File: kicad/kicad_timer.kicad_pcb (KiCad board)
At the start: 2 copper layers, 70.8 x 70.8 mm, 18 parts, among them J1 USB_C_Receptacle_PowerOnly_6P, U1 CA56-12CGKWA, U2 ATmega328-A, U3 CA56-12CGKWA

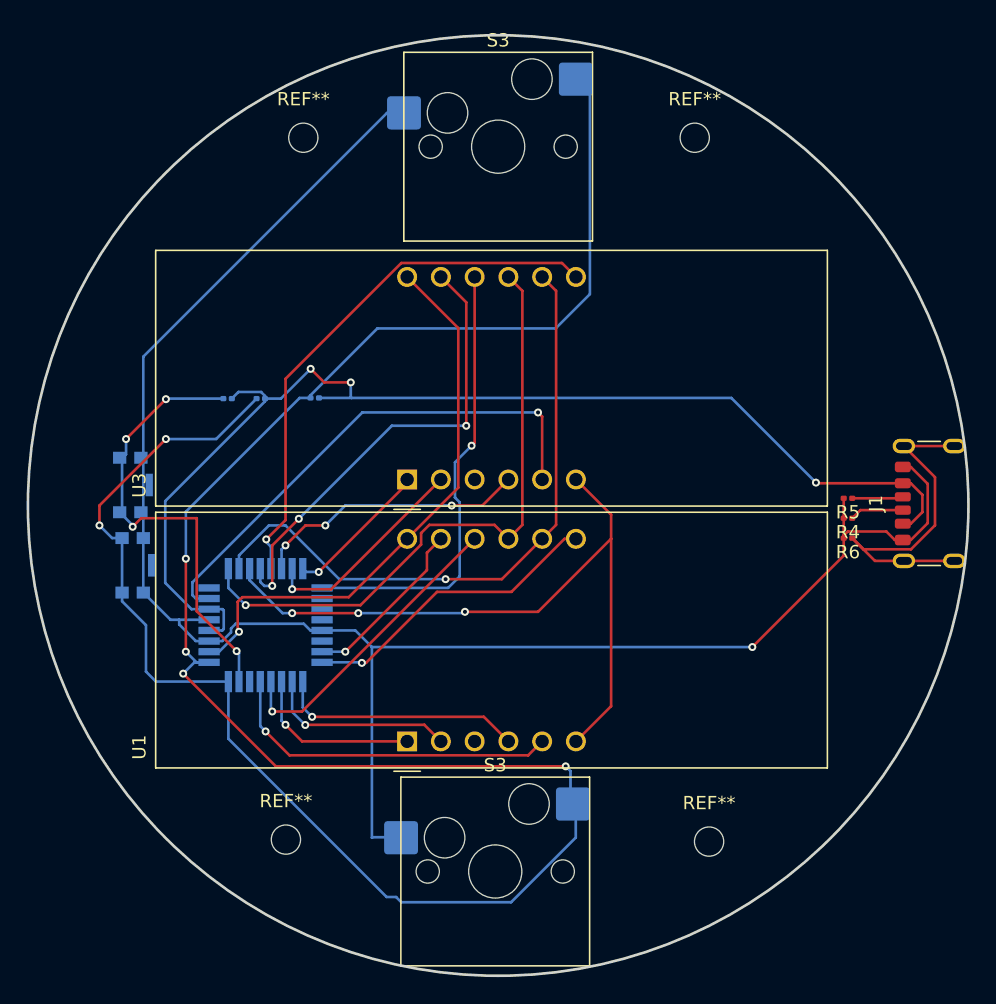
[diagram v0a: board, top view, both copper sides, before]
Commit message: Improving the pcb
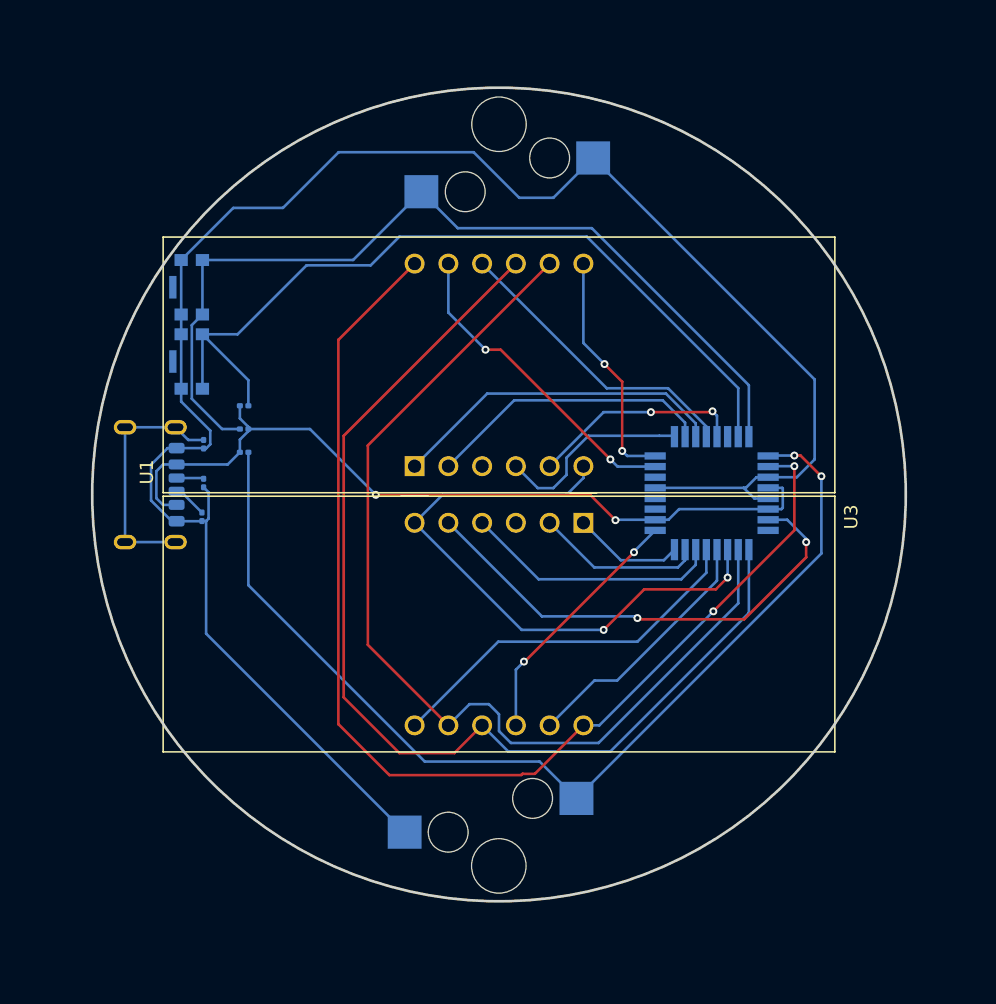
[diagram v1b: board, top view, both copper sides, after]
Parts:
- removed REF** (x4): MountingHole_2.2mm_M2_DIN965, MountingHole:MountingHole_2.2mm_M2_DIN965
- removed the S3 at (158.0, 123.1)
- removed the S3 at (158.2, 68.5)
- added S2: Keyswitch, kbd:keyswitch_cherrymx_hotswap_1u, B.Cu at (158.2, 66.9)
- added S3: Keyswitch, kbd:keyswitch_cherrymx_hotswap_1u, B.Cu at (158.2, 122.7)
- J1: moved to B.Cu
- R1, R2, R3: value Resistor -> 1K
- R4, R5: value Resistor -> 5.11 K; moved to B.Cu
- R6: value Resistor -> 1M resistor; moved to B.Cu
- moved J1 60.8 mm to (130.9, 94.0)
- moved R6 49.0 mm to (136.0, 90.9), turned to -90 degrees
- moved R4 48.6 mm to (135.9, 96.4), turned to -90 degrees
- moved R5 48.5 mm to (136.0, 93.9), turned to -90 degrees
- moved U2 35.0 mm to (174.2, 94.6), turned to 180 degrees
- moved S4 21.4 mm to (135.1, 79.1), turned to -90 degrees
- moved U1 20.7 mm to (151.9, 92.6)
- moved U3 13.7 mm to (164.6, 96.8), turned to -90 degrees
- moved S1 10.4 mm to (135.1, 84.7), turned to -90 degrees
- moved R3 6.71 mm to (139.1, 91.5), turned to 180 degrees
- moved R2 2.61 mm to (139.1, 89.8)
- moved R1 1.36 mm to (139.1, 88.0), turned to 180 degrees
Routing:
- net DIG1: track 42.8 -> 87.4 mm, vias 1 -> 2
- net DIG2: track 47.1 -> 81.0 mm, vias 1 -> 0
- net D1: track 34.4 -> 62.6 mm, vias 4 -> 0
- net Vcc: track 88.4 -> 60.7 mm, vias 3 -> 2
- net DIG3: track 48.2 -> 75.7 mm, vias 1 -> 0
- net D3: track 103.5 -> 77.9 mm, vias 4 -> 2
- net Net-(U2-PB0): track 35.4 -> 19.4 mm, vias 3 -> 0
- net Net-(U2-PB5): track 34.0 -> 19.0 mm, vias 1 -> 2
- net Net-(U2-PB1): track 40.9 -> 28.4 mm, vias 1 -> 0
- net Net-(U1-e): track 13.0 -> 25.3 mm, vias 1 -> 0
- net Net-(U1-a): track 13.2 -> 24.0 mm, vias 1 -> 2
- net Net-(U1-g): track 25.9 -> 16.0 mm, vias 1 -> 2
- net Net-(J1-SHIELD): track 26.6 -> 18.7 mm
- net DIG4: track 53.3 -> 45.6 mm, vias 3 -> 2
- net D2: track 76.1 -> 68.5 mm, vias 2 -> 0
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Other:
- board size 70.8 x 70.8 mm -> 61.2 x 61.2 mm
